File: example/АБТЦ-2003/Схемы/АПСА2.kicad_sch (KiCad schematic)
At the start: 34 parts

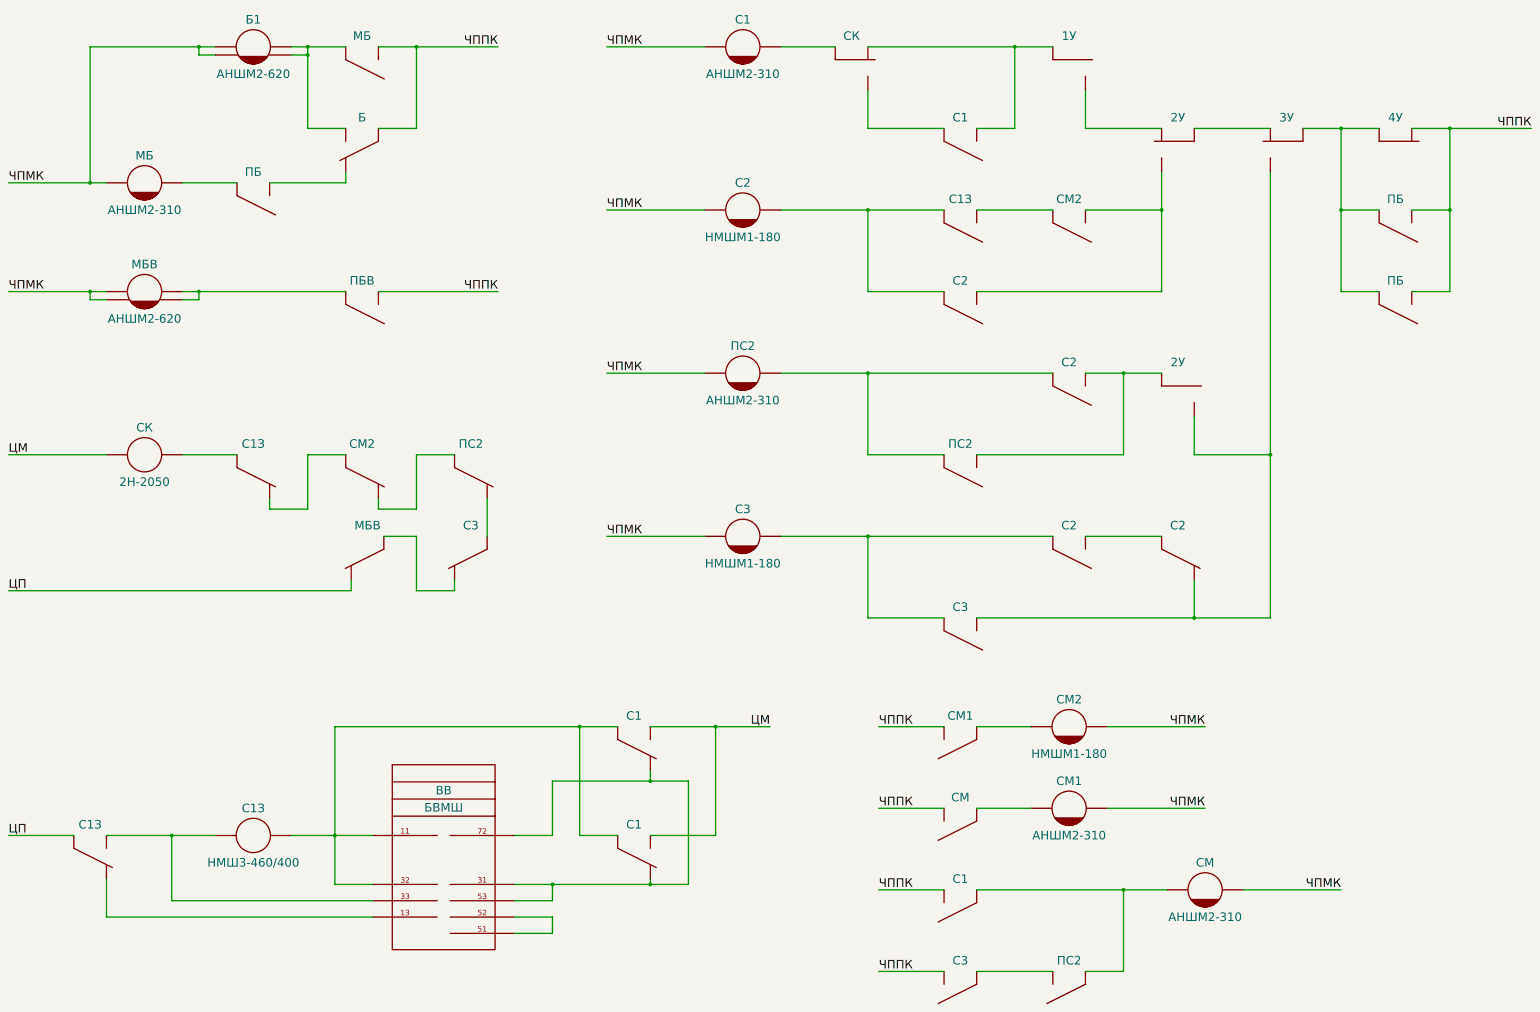
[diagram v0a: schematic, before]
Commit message: Шаблон АБТЦ обновлен
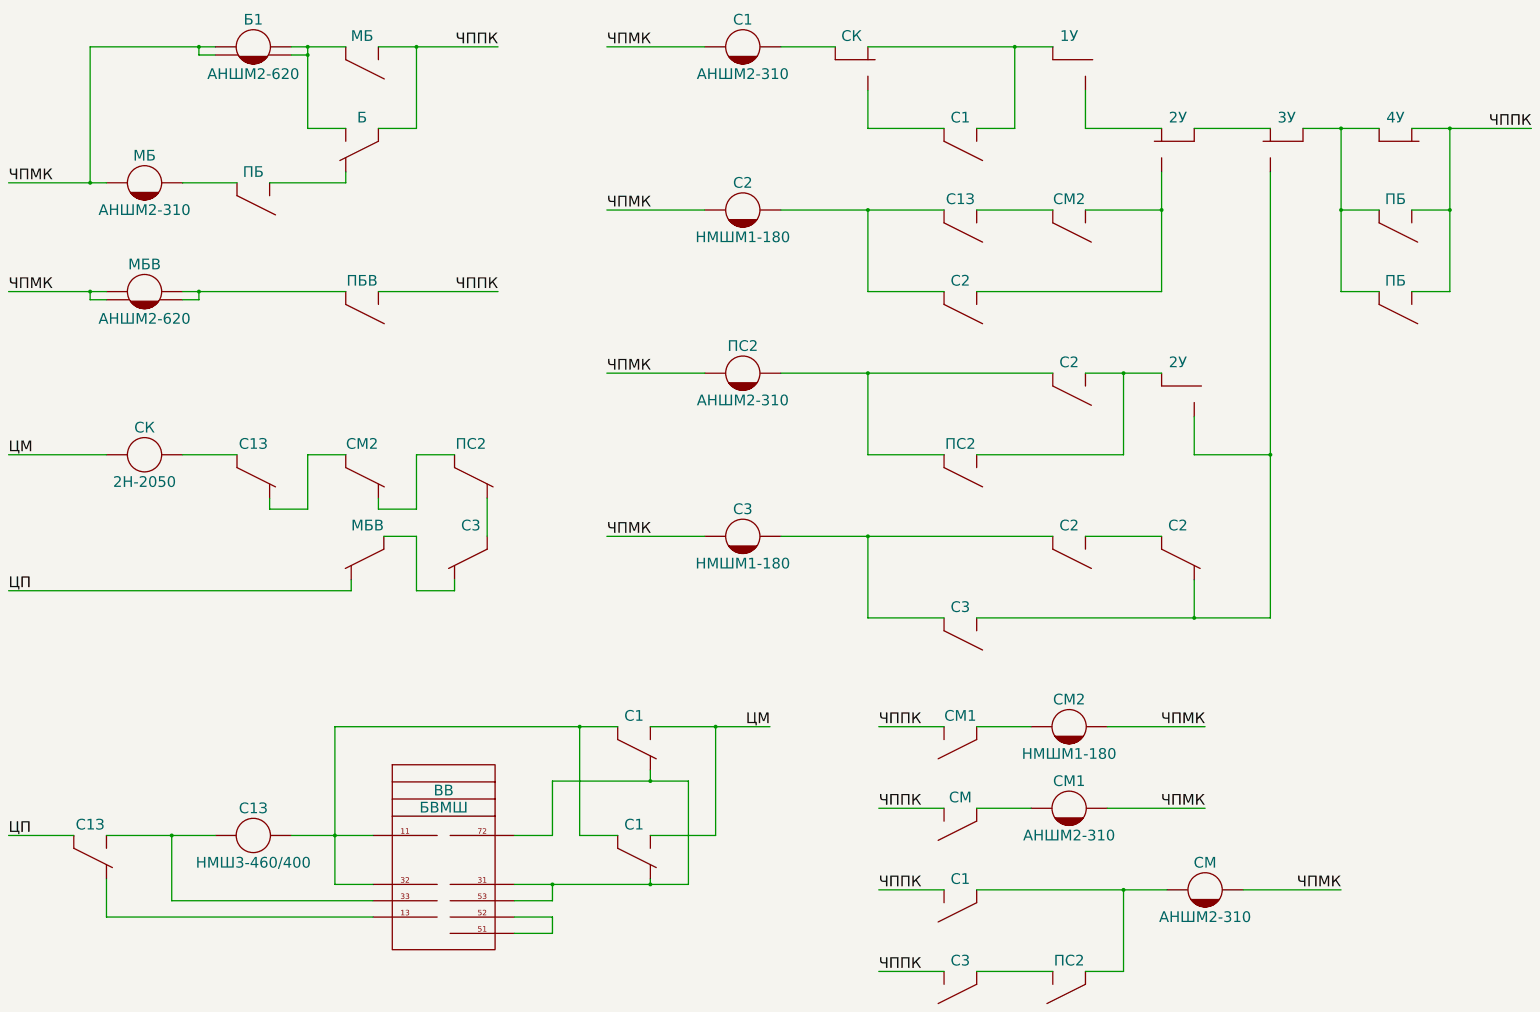
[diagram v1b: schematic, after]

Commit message: Обновление примера
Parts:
- Н1, Н11, Н111, Н1111, Н11111, Н111111, Н1111111, Н11111111, Н11112, Н111121, Н1111211, Н11112111: symbol SCB_Relay:Контакт_нейтрального_якоря -> SCB_Legacy:Контакт_нейтрального_якоря_бн
- Н11, Н111, Н13: symbol SCB_Relay:Контакт_нейтрального_якоря_НЗ -> SCB_Legacy:Контакт_нейтрального_якоря_НЗ_бн
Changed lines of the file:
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@@
 (kicad_sch
-	(version 20231120)
+	(version 20250114)
 	(generator "eeschema")
-	(generator_version "8.0")
+	(generator_version "9.0")
 	(paper "A3")
 	(title_block
@@
 	)
 	(symbol
-		(lib_id "SCB_Relay:Контакт_нейтрального_якоря_НЗ")
+		(lib_name "Контакт_нейтрального_якоря_НЗ_бн_2")
+		(lib_id "SCB_Legacy:Контакт_нейтрального_якоря_НЗ_бн")
 		(at 336.55 50.8 0)
 		(mirror y)
@@
 	)
 	(symbol
-		(lib_id "SCB_Relay:Контакт_нейтрального_якоря")
+		(lib_name "Контакт_нейтрального_якоря_бн_3")
+		(lib_id "SCB_Legacy:Контакт_нейтрального_якоря_бн")
 		(at 146.05 146.05 0)
 		(mirror y)
@@
 	)
 	(symbol
-		(lib_name "SCB_Relay:Контакт_нейтрального_якоря")
-		(lib_id "SCB_Relay:Контакт_нейтрального_якоря")
+		(lib_name "Контакт_нейтрального_якоря_бн_26")
+		(lib_id "SCB_Legacy:Контакт_нейтрального_якоря_бн")
 		(at 260.35 247.65 0)
 		(mirror y)
@@
 	)
 	(symbol
-		(lib_name "SCB_Relay:Контакт_нейтрального_якоря")
-		(lib_id "SCB_Relay:Контакт_нейтрального_якоря")
+		(lib_name "Контакт_нейтрального_якоря_бн_13")
+		(lib_id "SCB_Legacy:Контакт_нейтрального_якоря_бн")
 		(at 184.15 190.5 0)
 		(unit 1)
@@
 	)
 	(symbol
-		(lib_name "SCB_Relay:Контакт_нейтрального_якоря")
-		(lib_id "SCB_Relay:Контакт_нейтрального_якоря")
+		(lib_name "Контакт_нейтрального_якоря_бн_10")
+		(lib_id "SCB_Legacy:Контакт_нейтрального_якоря_бн")
 		(at 260.35 69.85 0)
 		(unit 3)
@@
 	)
 	(symbol
-		(lib_name "SCB_Relay:Контакт_нейтрального_якоря")
-		(lib_id "SCB_Relay:Контакт_нейтрального_якоря")
+		(lib_name "Контакт_нейтрального_якоря_бн_17")
+		(lib_id "SCB_Legacy:Контакт_нейтрального_якоря_бн")
 		(at 120.65 127 0)
 		(unit 2)
@@
 	)
 	(symbol
-		(lib_name "SCB_Relay:Контакт_нейтрального_якоря")
-		(lib_id "SCB_Relay:Контакт_нейтрального_якоря")
+		(lib_name "Контакт_нейтрального_якоря_бн_20")
+		(lib_id "SCB_Legacy:Контакт_нейтрального_якоря_бн")
 		(at 260.35 209.55 0)
 		(mirror y)
@@
 	)
 	(symbol
-		(lib_name "SCB_Relay:Контакт_нейтрального_якоря")
-		(lib_id "SCB_Relay:Контакт_нейтрального_якоря")
+		(lib_name "Контакт_нейтрального_якоря_бн_22")
+		(lib_id "SCB_Legacy:Контакт_нейтрального_якоря_бн")
 		(at 95.25 63.5 0)
 		(unit 3)
@@
 	)
 	(symbol
-		(lib_name "SCB_Relay:Контакт_нейтрального_якоря")
-		(lib_id "SCB_Relay:Контакт_нейтрального_якоря")
+		(lib_name "Контакт_нейтрального_якоря_бн_7")
+		(lib_id "SCB_Legacy:Контакт_нейтрального_якоря_бн")
 		(at 120.65 50.8 0)
 		(mirror y)
@@
 	)
 	(symbol
-		(lib_name "SCB_Relay:Контакт_нейтрального_якоря")
-		(lib_id "SCB_Relay:Контакт_нейтрального_якоря")
+		(lib_name "Контакт_нейтрального_якоря_бн_23")
+		(lib_id "SCB_Legacy:Контакт_нейтрального_якоря_бн")
 		(at 285.75 69.85 0)
 		(unit 3)
@@
 	)
 	(symbol
-		(lib_name "SCB_Relay:Контакт_нейтрального_якоря_НЗ")
-		(lib_id "SCB_Relay:Контакт_нейтрального_якоря_НЗ")
+		(lib_name "Контакт_нейтрального_якоря_НЗ_бн_3")
+		(lib_id "SCB_Legacy:Контакт_нейтрального_якоря_НЗ_бн")
 		(at 361.95 50.8 0)
 		(unit 3)
@@
 	)
 	(symbol
-		(lib_name "SCB_Relay:Контакт_нейтрального_якоря")
-		(lib_id "SCB_Relay:Контакт_нейтрального_якоря")
+		(lib_name "Контакт_нейтрального_якоря_бн_27")
+		(lib_id "SCB_Legacy:Контакт_нейтрального_якоря_бн")
 		(at 285.75 247.65 0)
 		(mirror y)
@@
 	)
 	(symbol
-		(lib_name "SCB_Relay:Контакт_нейтрального_якоря")
-		(lib_id "SCB_Relay:Контакт_нейтрального_якоря")
+		(lib_name "Контакт_нейтрального_якоря_бн_5")
+		(lib_id "SCB_Legacy:Контакт_нейтрального_якоря_бн")
 		(at 120.65 31.75 0)
 		(unit 3)
@@
 	)
 	(symbol
-		(lib_name "SCB_Relay:Контакт_нейтрального_якоря")
-		(lib_id "SCB_Relay:Контакт_нейтрального_якоря")
+		(lib_name "Контакт_нейтрального_якоря_бн_21")
+		(lib_id "SCB_Legacy:Контакт_нейтрального_якоря_бн")
 		(at 361.95 69.85 0)
 		(unit 3)
@@
 	)
 	(symbol
-		(lib_name "SCB_Relay:Контакт_нейтрального_якоря")
-		(lib_id "SCB_Relay:Контакт_нейтрального_якоря")
+		(lib_name "Контакт_нейтрального_якоря_бн_15")
+		(lib_id "SCB_Legacy:Контакт_нейтрального_якоря_бн")
 		(at 121.92 146.05 0)
 		(mirror y)
@@
 	)
 	(symbol
-		(lib_name "SCB_Relay:Контакт_нейтрального_якоря")
-		(lib_id "SCB_Relay:Контакт_нейтрального_якоря")
+		(lib_name "Контакт_нейтрального_якоря_бн_16")
+		(lib_id "SCB_Legacy:Контакт_нейтрального_якоря_бн")
 		(at 361.95 88.9 0)
 		(unit 3)
@@
 	)
 	(symbol
-		(lib_name "SCB_Relay:Контакт_нейтрального_якоря")
-		(lib_id "SCB_Relay:Контакт_нейтрального_якоря")
+		(lib_name "Контакт_нейтрального_якоря_бн_18")
+		(lib_id "SCB_Legacy:Контакт_нейтрального_якоря_бн")
 		(at 260.35 190.5 0)
 		(mirror y)
@@
 	)
 	(symbol
-		(lib_name "SCB_Relay:Контакт_нейтрального_якоря_НЗ")
-		(lib_id "SCB_Relay:Контакт_нейтрального_якоря_НЗ")
+		(lib_name "Контакт_нейтрального_якоря_НЗ_бн_5")
+		(lib_id "SCB_Legacy:Контакт_нейтрального_якоря_НЗ_бн")
 		(at 285.75 31.75 0)
 		(unit 2)
@@
 	)
 	(symbol
-		(lib_name "SCB_Relay:Контакт_нейтрального_якоря")
-		(lib_id "SCB_Relay:Контакт_нейтрального_якоря")
+		(lib_name "Контакт_нейтрального_якоря_бн_24")
+		(lib_id "SCB_Legacy:Контакт_нейтрального_якоря_бн")
 		(at 260.35 127 0)
 		(unit 3)
@@
 	)
 	(symbol
-		(lib_name "SCB_Relay:Контакт_нейтрального_якоря")
-		(lib_id "SCB_Relay:Контакт_нейтрального_якоря")
+		(lib_name "Контакт_нейтрального_якоря_бн_9")
+		(lib_id "SCB_Legacy:Контакт_нейтрального_якоря_бн")
 		(at 57.15 215.9 0)
 		(unit 1)
@@
 	)
 	(symbol
-		(lib_name "SCB_Relay:Контакт_нейтрального_якоря")
-		(lib_id "SCB_Relay:Контакт_нейтрального_якоря")
+		(lib_name "Контакт_нейтрального_якоря_бн_25")
+		(lib_id "SCB_Legacy:Контакт_нейтрального_якоря_бн")
 		(at 260.35 228.6 0)
 		(mirror y)
@@
 	)
 	(symbol
-		(lib_name "SCB_Relay:Контакт_нейтрального_якоря_НЗ")
-		(lib_id "SCB_Relay:Контакт_нейтрального_якоря_НЗ")
+		(lib_name "Контакт_нейтрального_якоря_НЗ_бн_4")
+		(lib_id "SCB_Legacy:Контакт_нейтрального_якоря_НЗ_бн")
 		(at 234.95 31.75 0)
 		(unit 1)
@@
 	)
 	(symbol
-		(lib_name "SCB_Relay:Контакт_нейтрального_якоря")
-		(lib_id "SCB_Relay:Контакт_нейтрального_якоря")
+		(lib_name "Контакт_нейтрального_якоря_бн_8")
+		(lib_id "SCB_Legacy:Контакт_нейтрального_якоря_бн")
 		(at 260.35 165.1 0)
 		(unit 3)
@@
 	)
 	(symbol
-		(lib_name "SCB_Relay:Контакт_нейтрального_якоря")
-		(lib_id "SCB_Relay:Контакт_нейтрального_якоря")
+		(lib_name "Контакт_нейтрального_якоря_бн_6")
+		(lib_id "SCB_Legacy:Контакт_нейтрального_якоря_бн")
 		(at 120.65 88.9 0)
 		(unit 3)
@@
 	)
 	(symbol
-		(lib_name "SCB_Relay:Контакт_нейтрального_якоря")
-		(lib_id "SCB_Relay:Контакт_нейтрального_якоря")
+		(lib_name "Контакт_нейтрального_якоря_бн_19")
+		(lib_id "SCB_Legacy:Контакт_нейтрального_якоря_бн")
 		(at 285.75 107.95 0)
 		(unit 3)
@@
 	)
 	(symbol
-		(lib_name "SCB_Relay:Контакт_нейтрального_якоря")
-		(lib_id "SCB_Relay:Контакт_нейтрального_якоря")
+		(lib_id "SCB_Legacy:Контакт_нейтрального_якоря_бн")
 		(at 285.75 146.05 0)
 		(unit 3)
@@
 	)
 	(symbol
-		(lib_name "SCB_Relay:Контакт_нейтрального_якоря")
-		(lib_id "SCB_Relay:Контакт_нейтрального_якоря")
+		(lib_name "Контакт_нейтрального_якоря_бн_1")
+		(lib_id "SCB_Legacy:Контакт_нейтрального_якоря_бн")
 		(at 311.15 146.05 0)
 		(unit 2)
@@
 	)
 	(symbol
-		(lib_name "SCB_Relay:Контакт_нейтрального_якоря")
-		(lib_id "SCB_Relay:Контакт_нейтрального_якоря")
+		(lib_name "Контакт_нейтрального_якоря_бн_14")
+		(lib_id "SCB_Legacy:Контакт_нейтрального_якоря_бн")
 		(at 260.35 88.9 0)
 		(unit 3)
@@
 	)
 	(symbol
-		(lib_name "SCB_Relay:Контакт_нейтрального_якоря")
-		(lib_id "SCB_Relay:Контакт_нейтрального_якоря")
+		(lib_name "Контакт_нейтрального_якоря_бн_4")
+		(lib_id "SCB_Legacy:Контакт_нейтрального_якоря_бн")
 		(at 95.25 127 0)
 		(unit 2)
@@
 	)
 	(symbol
-		(lib_name "SCB_Relay:Контакт_нейтрального_якоря")
-		(lib_id "SCB_Relay:Контакт_нейтрального_якоря")
+		(lib_name "Контакт_нейтрального_якоря_бн_2")
+		(lib_id "SCB_Legacy:Контакт_нейтрального_якоря_бн")
 		(at 260.35 50.8 0)
 		(unit 3)
@@
 	)
 	(symbol
-		(lib_name "SCB_Relay:Контакт_нейтрального_якоря")
-		(lib_id "SCB_Relay:Контакт_нейтрального_якоря")
+		(lib_name "Контакт_нейтрального_якоря_бн_11")
+		(lib_id "SCB_Legacy:Контакт_нейтрального_якоря_бн")
 		(at 146.05 127 0)
 		(unit 2)
@@
 	)
 	(symbol
-		(lib_name "SCB_Relay:Контакт_нейтрального_якоря_НЗ")
-		(lib_id "SCB_Relay:Контакт_нейтрального_якоря_НЗ")
+		(lib_id "SCB_Legacy:Контакт_нейтрального_якоря_НЗ_бн")
 		(at 311.15 107.95 0)
 		(unit 2)
@@
 	)
 	(symbol
-		(lib_name "SCB_Relay:Контакт_нейтрального_якоря")
-		(lib_id "SCB_Relay:Контакт_нейтрального_якоря")
+		(lib_name "Контакт_нейтрального_якоря_бн_12")
+		(lib_id "SCB_Legacy:Контакт_нейтрального_якоря_бн")
 		(at 184.15 215.9 0)
 		(unit 1)
@@
 	)
 	(symbol
-		(lib_name "SCB_Relay:Контакт_нейтрального_якоря_НЗ")
-		(lib_id "SCB_Relay:Контакт_нейтрального_якоря_НЗ")
+		(lib_name "Контакт_нейтрального_якоря_НЗ_бн_1")
+		(lib_id "SCB_Legacy:Контакт_нейтрального_якоря_НЗ_бн")
 		(at 311.15 50.8 0)
 		(mirror y)
